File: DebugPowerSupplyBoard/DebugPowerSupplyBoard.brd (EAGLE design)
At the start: 160 x 100 mm, 281 parts, among them IC1 LD117AV33, IC2 7805T

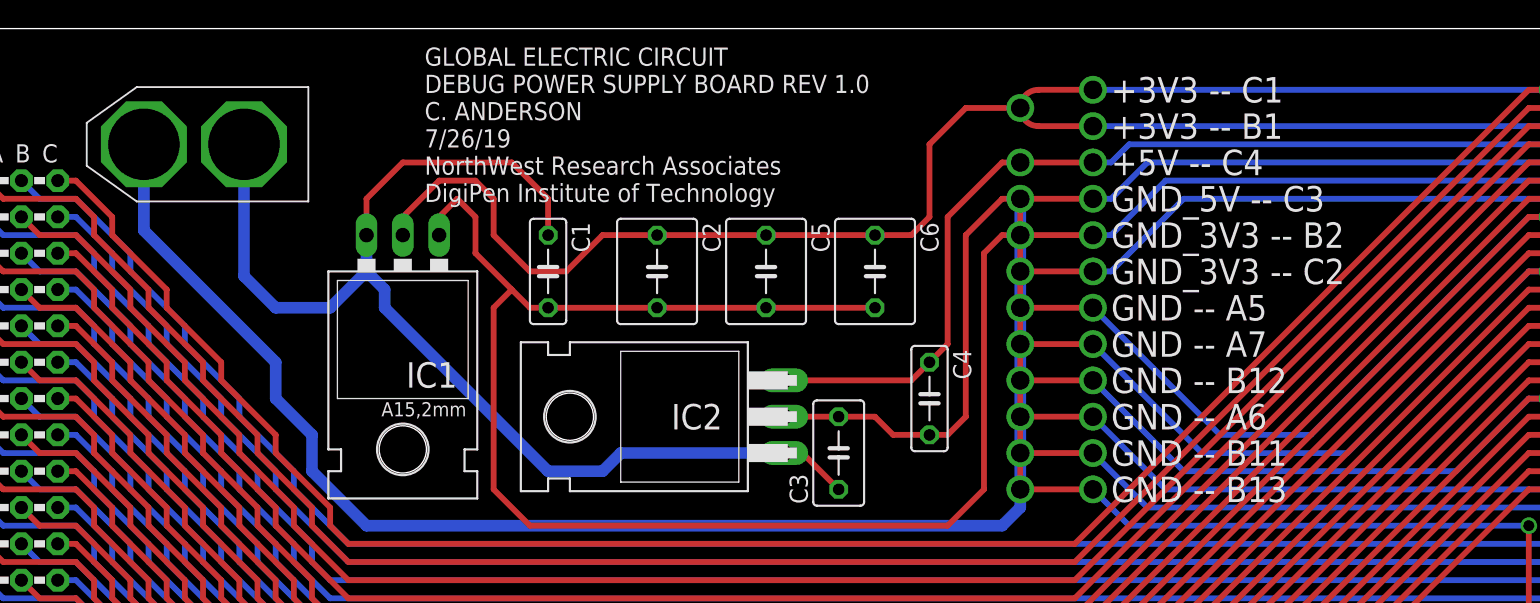
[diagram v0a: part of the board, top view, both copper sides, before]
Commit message: Alright, got it perfect, including adding a box around the board label ❤
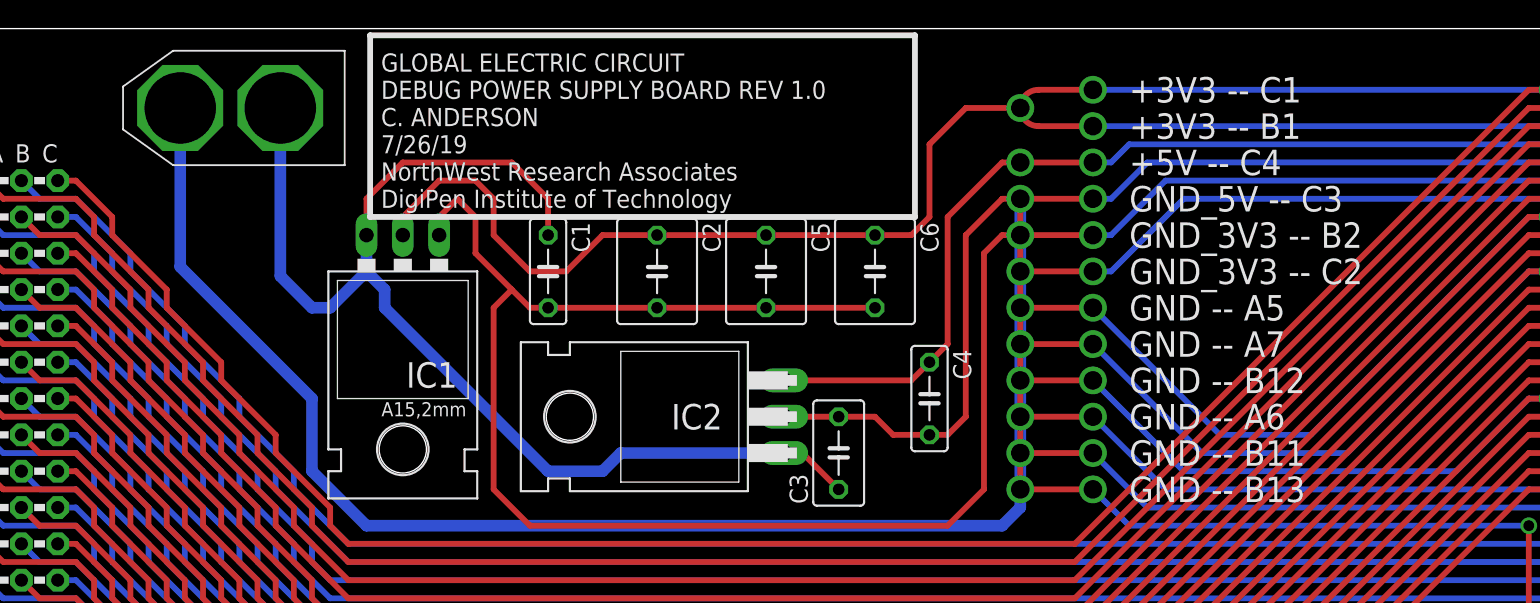
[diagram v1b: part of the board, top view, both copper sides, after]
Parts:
- moved U$6 3.59 mm to (30.2, 94.0)
- turned U$1 to 0 degrees
- turned U$10 to 0 degrees
- turned U$100 to 0 degrees
- turned U$101 to 0 degrees
- turned U$102 to 0 degrees
- turned U$103 to 0 degrees
- turned U$104 to 0 degrees
- turned U$105 to 0 degrees
- turned U$106 to 0 degrees
- turned U$107 to 0 degrees
- turned U$108 to 0 degrees
- turned U$109 to 0 degrees
- turned U$11 to 0 degrees
- turned U$110 to 0 degrees
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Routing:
- net GND: track 2259.9 -> 2261.4 mm
